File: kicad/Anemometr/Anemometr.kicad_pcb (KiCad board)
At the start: 2 copper layers, 44.9 x 45.2 mm, 162 parts, among them J10 +Z3, J11 -Z3, J12 +Z4, J13 -Z4, J14 SWD, J15 SWC, J18 1 TxD+, J19 2 TxD-, J2 Conn_01x01_Female, J20 3 RxD+, J21 4-5, J23 6 RxD-, J24 7-8, J3 RST, J36 TMP117, J37 TMP117, J38 TMP117, J39 TMP117, J4 TxD, J5 RxD, J6 +Z1, J7 -Z1, J8 +Z2, J9 -Z2, Q1 5N10, U1 TS5A3166DBVR, U10 MCP1700-3002E, U2 LMV7239, U3 TS5A3166DBVR, U4 TS5A3166DBVR, U5 STM32F103C8Tx, U6 TS5A3166DBVR, U7 LM2734Y, U8 MCP1700-5002E, U9 MCP1700-3002E, Y1 8MHz, Y2 25MHz

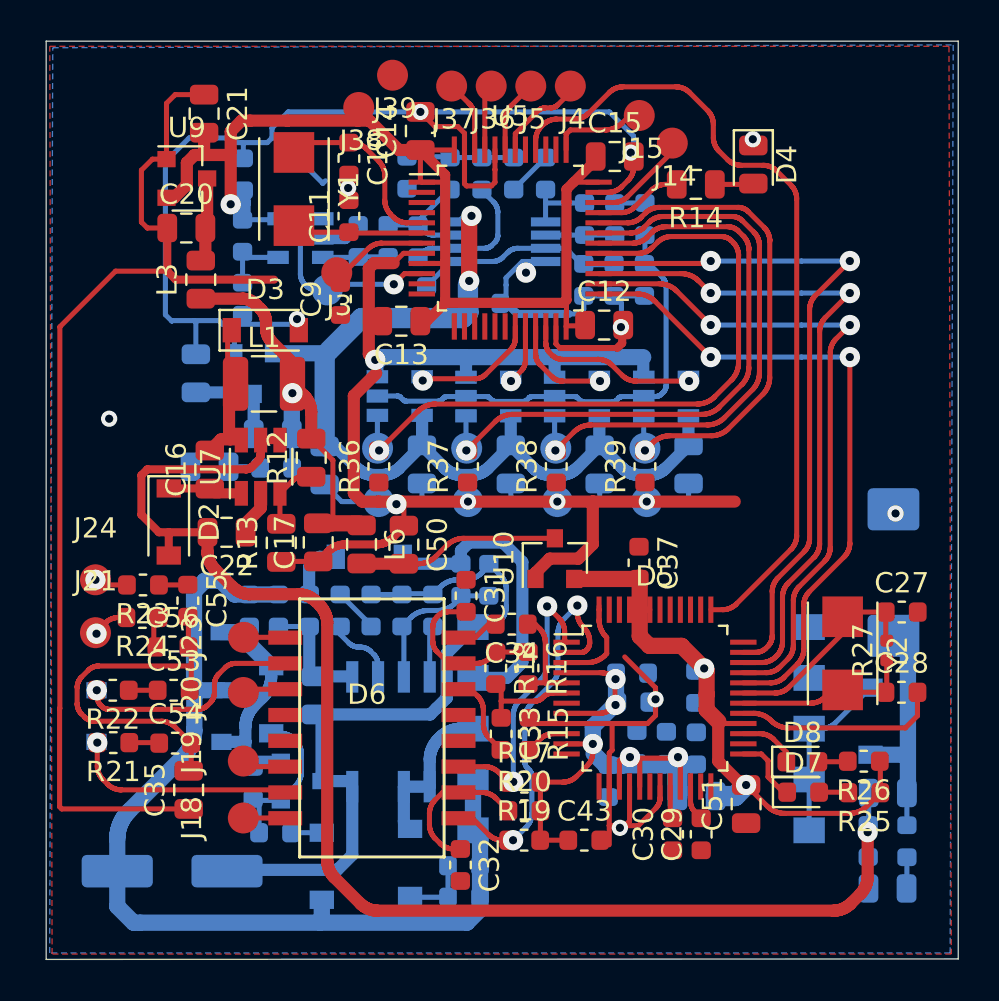
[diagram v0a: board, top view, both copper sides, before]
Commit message: изменено:      FreeCAD/base-4.FCStd 	изменено:      FreeCAD/base-4.stl 	изменено:      FreeCAD/cover-4.fcstd 	изменено:      FreeCAD/cover-4.stl 	изменено:      FreeCAD/holder-3.fcstd 	изменено:      kicad/Anemometr/Anemometr.kicad_pcb 	изменено:      kicad/Anemometr/Anemometr.kicad_pcb-bak 	изменено:      kicad/Anemometr/Anemometr.sch 	изменено:      kicad/Anemometr/Anemometr.sch-bak
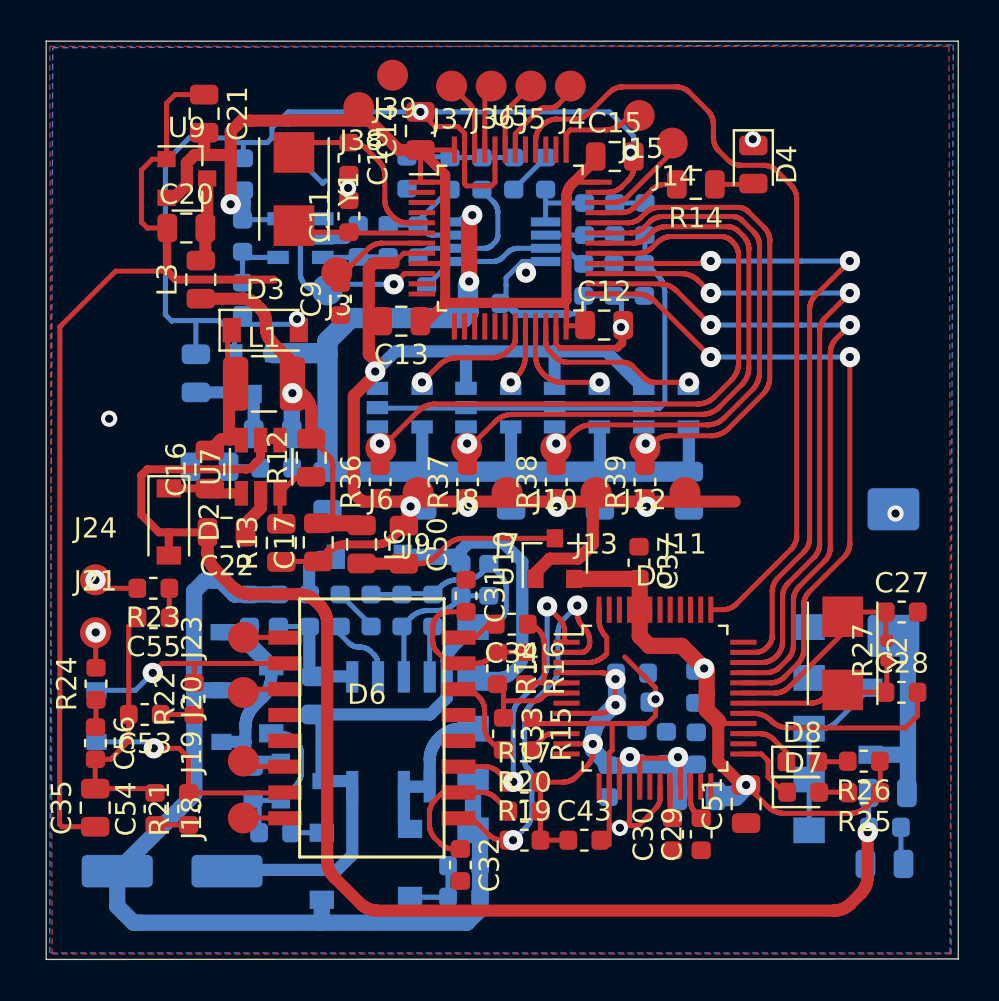
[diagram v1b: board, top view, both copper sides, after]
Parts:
- removed R35: 2k, Resistor_SMD:R_0603_1608Metric
- J10, J11, J12, J13, J6, J7, J8, J9: moved to F.Cu
- moved C56 6.06 mm to (21.3, 94.1), turned to 270 degrees
- moved R21 4.94 mm to (25.9, 97.4), turned to 90 degrees
- moved C35 4.68 mm to (21.3, 97.3)
- moved R22 4.02 mm to (26.1, 92.0), turned to 90 degrees
- moved R24 3.98 mm to (21.3, 91.2), turned to 90 degrees
- moved C54 3.39 mm to (24.2, 97.4), turned to 90 degrees
- moved J9 1.99 mm to (37.2, 81.8)
- moved J7 1.97 mm to (41.6, 81.8)
- moved J13 1.95 mm to (45.9, 81.8)
- moved J11 1.93 mm to (50.3, 81.8)
- moved C55 1.89 mm to (24.2, 88.0), turned to 180 degrees
- moved C53 1.86 mm to (23.7, 92.7), turned to 180 degrees
- moved C23 1.30 mm to (41.7, 81.7)
- moved C24 1.30 mm to (37.4, 81.7)
- moved C25 1.30 mm to (50.5, 81.7)
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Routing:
- net GND: track 261.6 -> 236.5 mm
- net Net-(C35-Pad2): track 18.7 -> 12.7 mm
- net Net-(C49-Pad1): track 11.6 -> 10.0 mm
- net Net-(D10-Pad2): track 1.65 -> 2.23 mm
- net Net-(D6-Pad10): track 11.3 -> 10.8 mm
